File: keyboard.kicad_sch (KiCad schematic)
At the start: 28 parts, among them J1 SSD1306, J2 Conn_01x05, J3 USB_C_Receptacle_USB2.0, SW1 RotaryEncoder_Switch, SW2 SW_Push, SW3 SW_Push, U1 STM32F072CBTx, U2 AMS1117-3.3, U3 SRV05-4

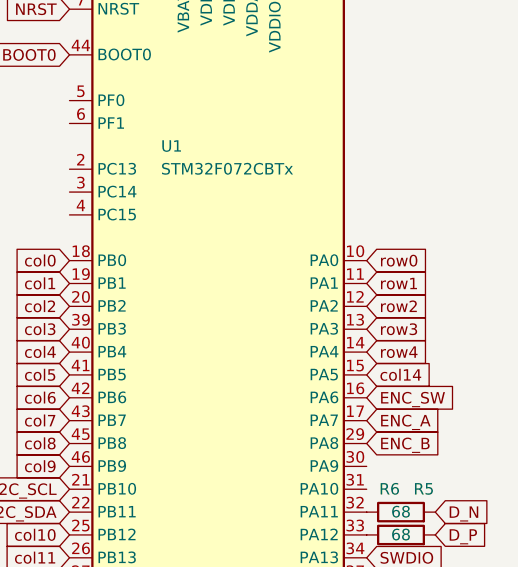
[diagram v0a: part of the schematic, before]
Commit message: more wiring done
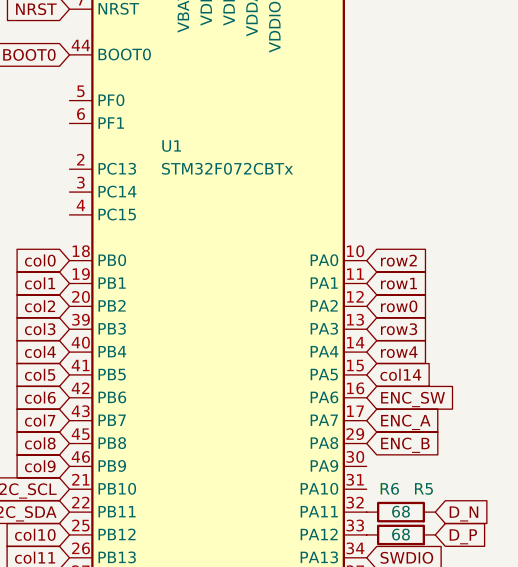
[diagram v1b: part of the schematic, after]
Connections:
- net row0: now also U1.12 (PA2); no longer U1.10 (PA0)
- net row2: now also U1.10 (PA0); no longer U1.12 (PA2)
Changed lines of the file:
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@@
     )
   )
-  (global_label "row0" (shape input) (at 266.7 110.49 0) (fields_autoplaced)
+  (global_label "row0" (shape input) (at 266.7 115.57 0) (fields_autoplaced)
     (effects (font (size 1.27 1.27)) (justify left))
-    (property "Intersheetrefs" "${INTERSHEET_REFS}" (at 273.5883 110.5694 0)
+    (property "Intersheetrefs" "${INTERSHEET_REFS}" (at 273.5883 115.6494 0)
       (effects (font (size 1.27 1.27)) (justify left) hide)
     )
@@
     )
   )
-  (global_label "row2" (shape input) (at 266.7 115.57 0) (fields_autoplaced)
+  (global_label "row2" (shape input) (at 266.7 110.49 0) (fields_autoplaced)
     (effects (font (size 1.27 1.27)) (justify left))
-    (property "Intersheetrefs" "${INTERSHEET_REFS}" (at 273.5883 115.6494 0)
+    (property "Intersheetrefs" "${INTERSHEET_REFS}" (at 273.5883 110.5694 0)
       (effects (font (size 1.27 1.27)) (justify left) hide)
     )

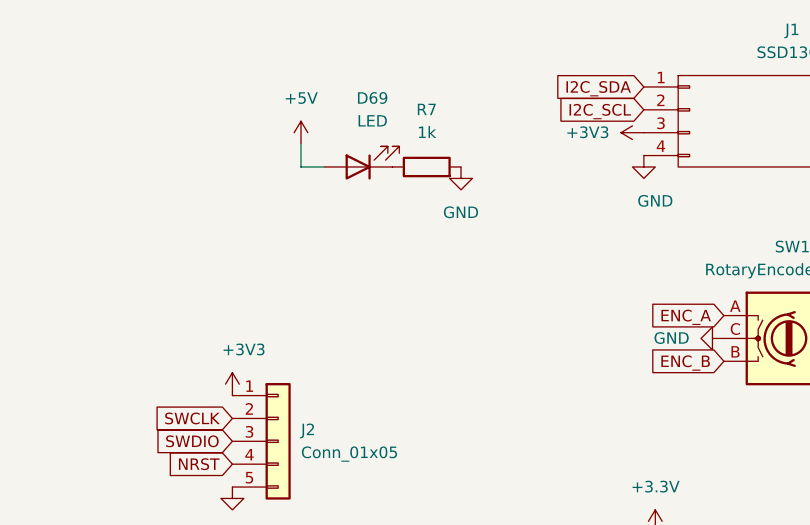
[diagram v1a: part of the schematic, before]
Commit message: nuked traces, start again
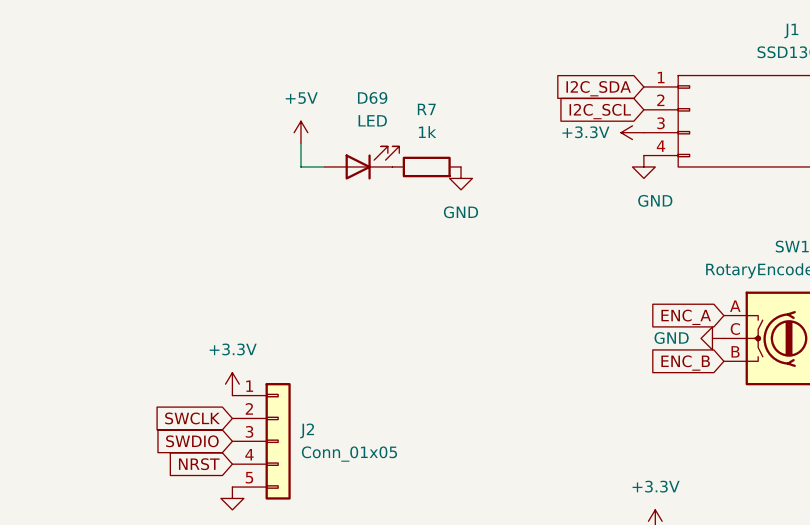
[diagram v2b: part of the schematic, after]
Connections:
- net +3V3 is gone; now on net +3.3V: J1.3 (VCC), J2.1 (Pin_1)
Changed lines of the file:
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@@
+    )
+  )
+  (symbol (lib_id "power:+3.3V") (at 199.39 59.69 0) (unit 1)
+    (in_bom yes) (on_board yes) (dnp no) (fields_autoplaced)
+    (property "Reference" "#PWR05" (at 199.39 63.5 0)
+      (effects (font (size 1.27 1.27)) hide)
+    )
+    (property "Value" "+3.3V" (at 199.39 54.61 0)
+      (effects (font (size 1.27 1.27)))
+    )
+    (property "Footprint" "" (at 199.39 59.69 0)
+      (effects (font (size 1.27 1.27)) hide)
+    )
+    (property "Datasheet" "" (at 199.39 59.69 0)
+      (effects (font (size 1.27 1.27)) hide)
+    )
+    (pin "1")
+    (instances
+      (project "keyboard"
+        (path "/34e6269a-59e1-46fb-8424-28258a1346a0"
+          (reference "#PWR05") (unit 1)
+        )
+      )
     )
   )
@@
     )
   )
+  (symbol (lib_id "power:+3.3V") (at 245.11 30.48 90) (unit 1)
+    (in_bom yes) (on_board yes) (dnp no) (fields_autoplaced)
+    (property "Reference" "#PWR06" (at 248.92 30.48 0)
+      (effects (font (size 1.27 1.27)) hide)
+    )
+    (property "Value" "+3.3V" (at 241.3 30.48 90)
+      (effects (font (size 1.27 1.27)) (justify left))
+    )
+    (property "Footprint" "" (at 245.11 30.48 0)
+      (effects (font (size 1.27 1.27)) hide)
+    )
+    (property "Datasheet" "" (at 245.11 30.48 0)
+      (effects (font (size 1.27 1.27)) hide)
+    )
+    (pin "1")
+    (instances
+      (project "keyboard"
+        (path "/34e6269a-59e1-46fb-8424-28258a1346a0"
+          (reference "#PWR06") (unit 1)
+        )
+      )
+    )
+  )
   (symbol (lib_id "Device:R") (at 220.98 34.29 90) (unit 1)
     (in_bom yes) (on_board yes) (dnp no) (fields_autoplaced)
@@
         (path "/34e6269a-59e1-46fb-8424-28258a1346a0"
           (reference "C_VDDA1") (unit 1)
-        )
-      )
-    )
-  )
-  (symbol (lib_id "power:+3V3") (at 245.11 30.48 90) (unit 1)
-    (in_bom yes) (on_board yes) (dnp no)
-    (property "Reference" "#PWR0101" (at 248.92 30.48 0)
-      (effects (font (size 1.27 1.27)) hide)
-    )
-    (property "Value" "+3V3" (at 241.3 30.48 90)
-      (effects (font (size 1.27 1.27)) (justify left))
-    )
-    (property "Footprint" "" (at 245.11 30.48 0)
-      (effects (font (size 1.27 1.27)) hide)
-    )
-    (property "Datasheet" "" (at 245.11 30.48 0)
-      (effects (font (size 1.27 1.27)) hide)
-    )
-    (pin "1")
-    (instances
-      (project "keyboard"
-        (path "/34e6269a-59e1-46fb-8424-28258a1346a0"
-          (reference "#PWR0101") (unit 1)
         )
       )
@@
         )
       )
-    )
-  )
-  (symbol (lib_id "power:+3V3") (at 199.39 59.69 0) (unit 1)
-    (in_bom yes) (on_board yes) (dnp no)
-    (property "Reference" "#PWR0106" (at 199.39 63.5 0)
-      (effects (font (size 1.27 1.27)) hide)
-    )
-    (property "Value" "+3V3" (at 200.66 54.61 0)
-      (effects (font (size 1.27 1.27)))
-    )
-    (property "Footprint" "" (at 199.39 59.69 0)
-      (effects (font (size 1.27 1.27)) hide)
-    )
-    (property "Datasheet" "" (at 199.39 59.69 0)
-      (effects (font (size 1.27 1.27)) hide)
-    )
-    (pin "1")
-    (instances
-      (project "keyboard"
-        (path "/34e6269a-59e1-46fb-8424-28258a1346a0"
-          (reference "#PWR0106") (unit 1)
-        )
-      )

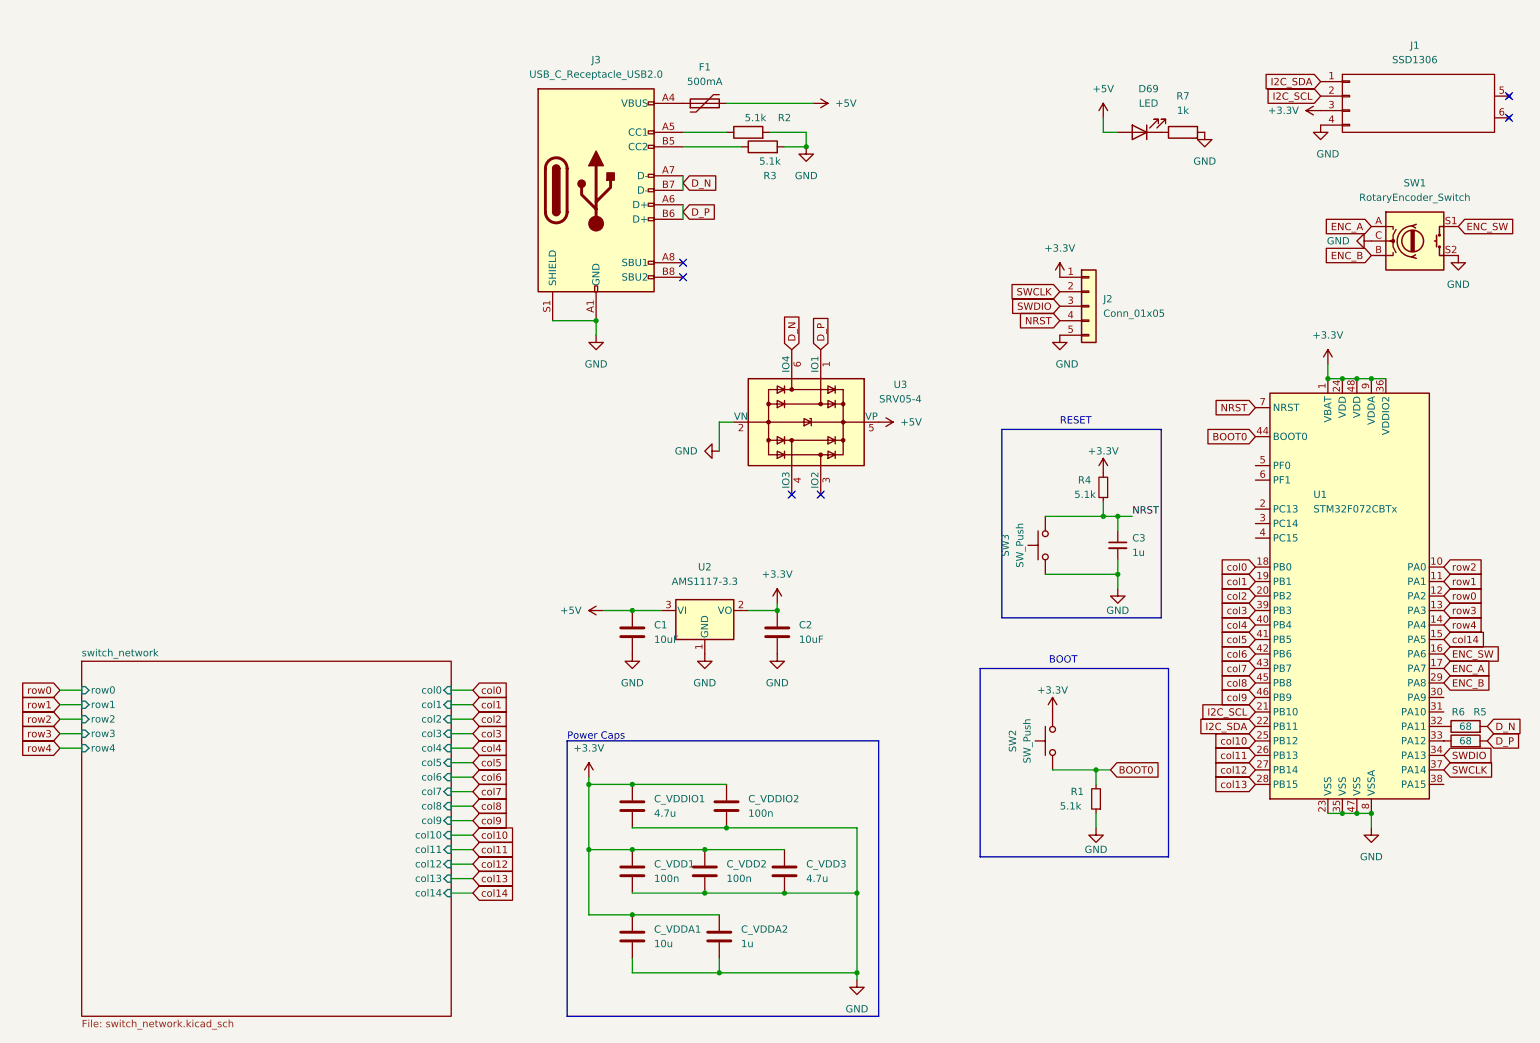
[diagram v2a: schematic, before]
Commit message: code?
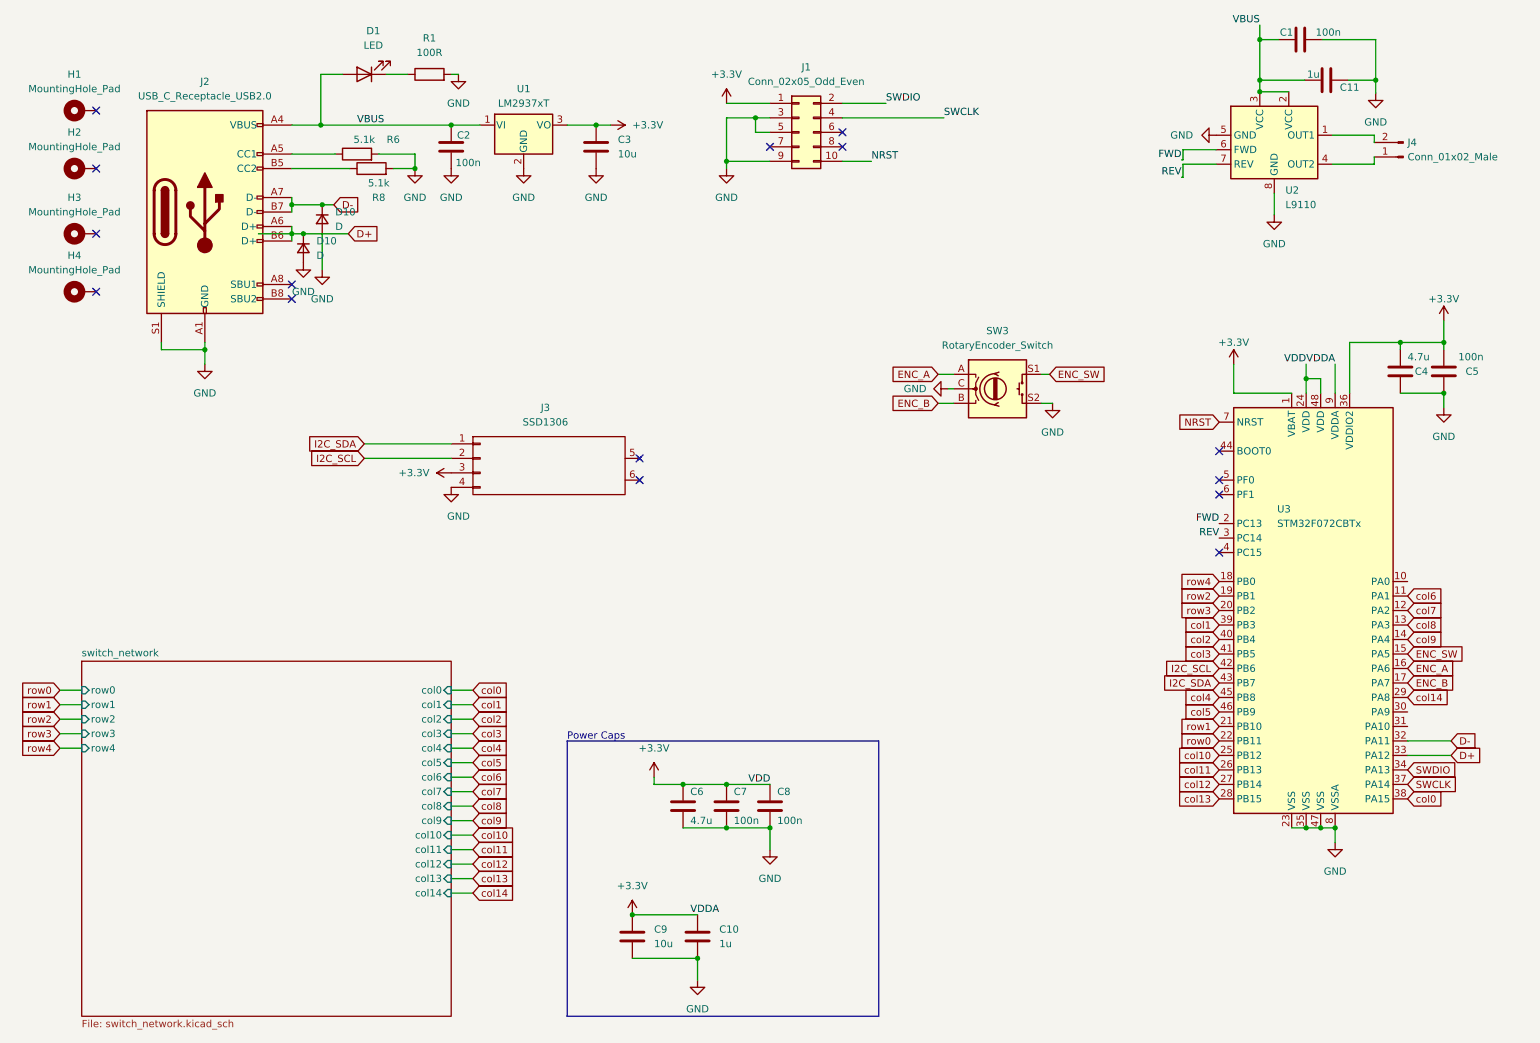
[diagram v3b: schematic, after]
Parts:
- removed C3: 1u, Capacitor_THT:CP_Radial_D4.0mm_P1.50mm, symbol Device:C_Small
- removed C_VDD1, C_VDD2, C_VDDIO2: 100n, Capacitor_THT:C_Disc_D5.0mm_W2.5mm_P2.50mm, symbol Device:C
- removed C_VDD3, C_VDDIO1: 4.7u, Capacitor_THT:CP_Radial_D4.0mm_P1.50mm, symbol Device:C
- removed F1: 500mA, marbastvary:polyfuse_5.1mm, symbol Device:Polyfuse
- removed J2: Conn_01x05, Connector_PinHeader_2.54mm:PinHeader_1x05_P2.54mm_Vertical, symbol Connector_Generic:Conn_01x05
- removed J3: USB_C_Receptacle_USB2.0, USB-C:TYPE-C-31-M-12, symbol Connector:USB_C_Receptacle_USB2.0
- removed R1, R4: 5.1k, Resistor_THT:R_Axial_DIN0204_L3.6mm_D1.6mm_P5.08mm_Horizontal, symbol Device:R_Small
- removed R5, R6: 68, Resistor_THT:R_Axial_DIN0204_L3.6mm_D1.6mm_P5.08mm_Horizontal, symbol Device:R
- removed SW2, SW3: SW_Push, Button_Switch_THT:SW_PUSH_6mm, symbol Switch:SW_Push
- removed U2: AMS1117-3.3, Package_TO_SOT_SMD:SOT-223-3_TabPin2, symbol Regulator_Linear:AMS1117-3.3
- removed U3: SRV05-4, marbastvary:SOT-23-6-routable, symbol marbastlib-various:SRV05-4
- added C1: 100n, Capacitor_SMD:C_0805_2012Metric, symbol Device:C
- added C11: 1u, Capacitor_SMD:C_0805_2012Metric, symbol Device:C
- added C4, C6: 4.7u, Capacitor_SMD:C_0805_2012Metric, symbol Device:C
- added C5, C7, C8: 100n, Capacitor_SMD:C_0603_1608Metric, symbol Device:C
- added D10 (x2): D, marbastvary:D_DO-35_SOD27_P5.08mm_Horizontal, symbol Device:D_Small
- added H1, H2, H3, H4: MountingHole_Pad, MountingHole:MountingHole_3.2mm_M3_Pad, symbol Mechanical:MountingHole_Pad
- added J1: Conn_02x05_Odd_Even, Connector:322010010000, symbol Connector_Generic:Conn_02x05_Odd_Even
- added J2: USB_C_Receptacle_USB2.0, Connector_USB:USB_C_Receptacle_G-Switch_GT-USB-7010ASV, symbol Connector:USB_C_Receptacle_USB2.0
- added J4: Conn_01x02_Male, Connector_PinHeader_2.54mm:PinHeader_1x02_P2.54mm_Vertical, symbol Connector:Conn_01x02_Male
- added U1: LM2937xT, Package_TO_SOT_THT:TO-220-3_Horizontal_TabDown, symbol Regulator_Linear:LM2937xT
- added U2: L9110, Package_DIP:DIP-8_W7.62mm, symbol Driver_Motor:ZXBM5210-S
- C10: renamed from C_VDDA2; footprint Capacitor_THT:CP_Radial_D4.0mm_P1.50mm -> Capacitor_SMD:C_0805_2012Metric
- C2: renamed from C1; value 10uF -> 100n; footprint Capacitor_THT:CP_Radial_D4.0mm_P1.50mm -> Capacitor_SMD:C_0805_2012Metric
- C3: renamed from C2; value 10uF -> 10u; footprint Capacitor_THT:CP_Radial_D4.0mm_P1.50mm -> Capacitor_SMD:C_0805_2012Metric
- C9: renamed from C_VDDA1; footprint Capacitor_THT:CP_Radial_D4.0mm_P1.50mm -> Capacitor_SMD:C_0805_2012Metric
- R1: renamed from R7; value 1k -> 100R; footprint Resistor_THT:R_Axial_DIN0204_L3.6mm_D1.6mm_P5.08mm_Horizontal -> Resistor_THT:R_Axial_DIN0207_L6.3mm_D2.5mm_P7.62mm_Horizontal
- R6: renamed from R2; footprint Resistor_THT:R_Axial_DIN0204_L3.6mm_D1.6mm_P5.08mm_Horizontal -> Resistor_THT:R_Axial_DIN0207_L6.3mm_D2.5mm_P7.62mm_Horizontal
- R8: renamed from R3; footprint Resistor_THT:R_Axial_DIN0204_L3.6mm_D1.6mm_P5.08mm_Horizontal -> Resistor_THT:R_Axial_DIN0207_L6.3mm_D2.5mm_P7.62mm_Horizontal
- renumbered D69 to D1, J1 to J3, SW1 to SW3, U1 to U3
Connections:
- net +3.3V: now also C4.1, C5.1, C6.1, C7.1, C8.1, J1.1 (Pin_1), U1.3 (VO)
- net ENC_A: now also U3.16 (PA6); no longer U3.17 (PA7)
- net ENC_B: now also U3.17 (PA7); no longer U3.29 (PA8)
- net ENC_SW: now also U3.15 (PA5); no longer U3.16 (PA6)
- net GND: now also C1.2, C11.2, C4.2, C5.2, C6.2, C7.2, C8.2, D10.2 (A), D10.2 (A), J1.3 (Pin_3), J1.5 (Pin_5), J1.9 (Pin_9), J2.A1 (GND), J2.A12 (GND), J2.B1 (GND), J2.B12 (GND), J2.S1 (SHIELD), U1.2 (GND), U2.5 (GND), U2.8 (GND)
- net I2C_SCL: now also U3.42 (PB6); no longer U3.21 (PB10)
- net I2C_SDA: now also U3.43 (PB7); no longer U3.22 (PB11)
- net NRST: now also J1.10 (Pin_10)
- net SWCLK: now also J1.4 (Pin_4)
- net SWDIO: now also J1.2 (Pin_2)
- net col0: now also U3.38 (PA15); no longer U3.18 (PB0)
- net col1: now also U3.39 (PB3); no longer U3.19 (PB1)
- net col14: now also U3.29 (PA8); no longer U3.15 (PA5)
- net col2: now also U3.40 (PB4); no longer U3.20 (PB2)
- net col3: now also U3.41 (PB5); no longer U3.39 (PB3)
- net col4: now also U3.45 (PB8); no longer U3.40 (PB4)
- net col5: now also U3.46 (PB9); no longer U3.41 (PB5)
- net col6: now also U3.11 (PA1); no longer U3.42 (PB6)
- net col7: now also U3.12 (PA2); no longer U3.43 (PB7)
- net col8: now also U3.13 (PA3); no longer U3.45 (PB8)
- net col9: now also U3.14 (PA4); no longer U3.46 (PB9)
- net row0: now also U3.22 (PB11); no longer U3.12 (PA2)
- net row1: now also U3.21 (PB10); no longer U3.11 (PA1)
- net row2: now also U3.19 (PB1); no longer U3.10 (PA0)
- net row3: now also U3.20 (PB2); no longer U3.13 (PA3)
- net row4: now also U3.18 (PB0); no longer U3.14 (PA4)
- net at R8.1: now also J2.B5 (CC2)
- net D+: now reaches U3.33 (PA12)
- net D+: now also D10.1 (K), J2.A6 (D+), J2.B6 (D+)
- net D-: now reaches U3.32 (PA11)
- net D-: now also D10.1 (K), J2.A7 (D-), J2.B7 (D-)
- net FWD: now reaches U3.2 (PC13)
- net FWD: now also U2.6 (FWD)
- net REV: now reaches U3.3 (PC14)
- net REV: now also U2.7 (REV)
- net at R6.1: now also J2.A5 (CC1)
- net +5V renamed VBUS
- net VBUS: now also C1.1, C11.1, J2.A4 (VBUS), J2.A9 (VBUS), J2.B4 (VBUS), J2.B9 (VBUS), U1.1 (VI), U2.2 (VCC), U2.3 (VCC)
- net BOOT0: no longer names the net of U3.44 (BOOT0)
- new net: J4.2 (Pin_2), U2.1 (OUT1)
- new net: J4.1 (Pin_1), U2.4 (OUT2)
- no-connect marks 6 -> 15
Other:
- note removed: "BOOT"
- note removed: "RESET"
- moved on the sheet: C10, C2, C3, D1, J3, R1, R6, R8, SW3, U3
